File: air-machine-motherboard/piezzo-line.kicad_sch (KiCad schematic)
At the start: 8 parts, among them J3 OUT, Q1 BU407

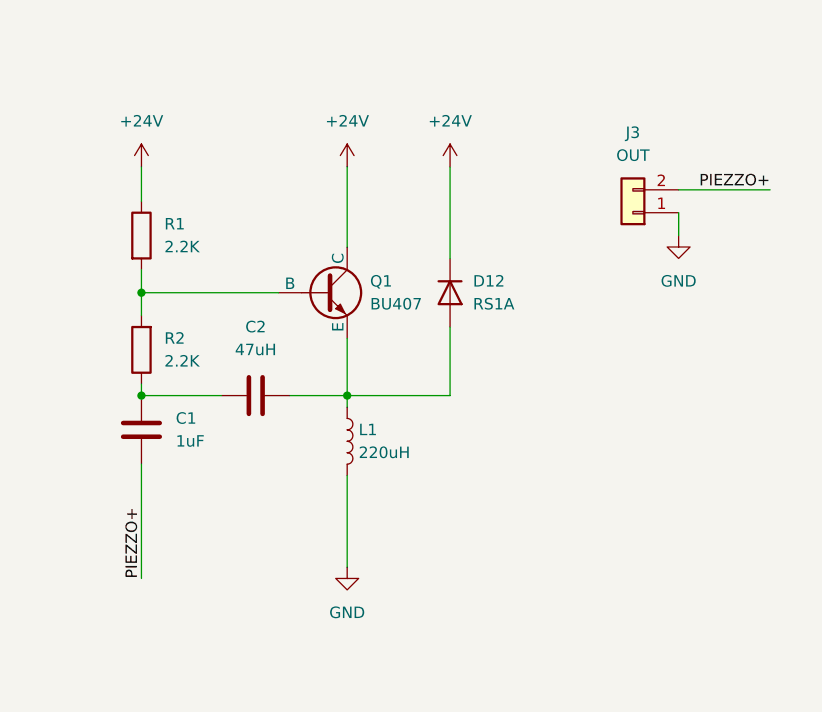
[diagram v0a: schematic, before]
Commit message: wireles air machine motherboard
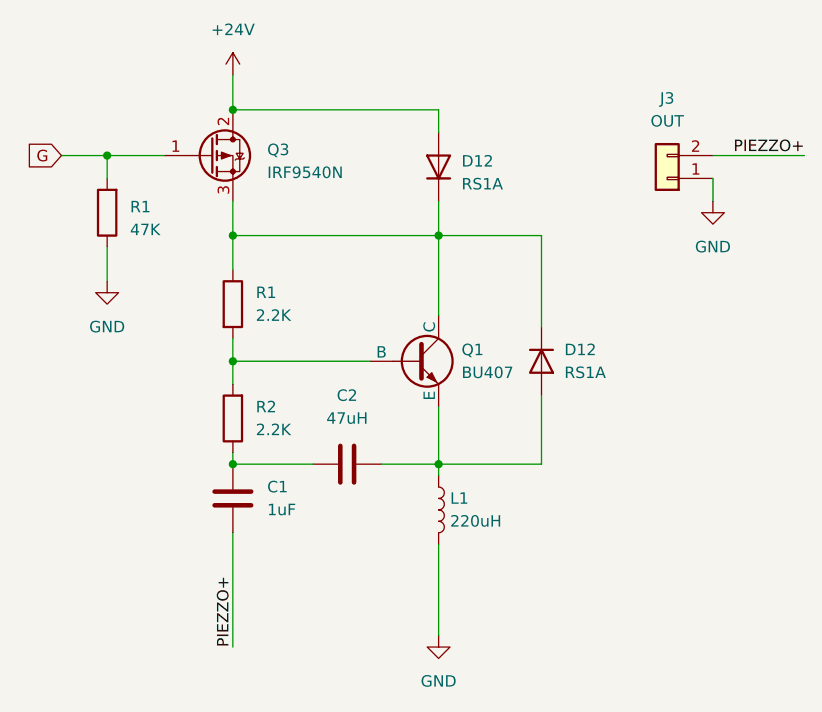
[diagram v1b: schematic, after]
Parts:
- added D12: RS1A, Diode_SMD:D_MELF, symbol Device:D
- added Q3: IRF9540N, Package_TO_SOT_THT:TO-220-3_Vertical, symbol Transistor_FET:IRF9540N
- added R1: 47K, Resistor_SMD:R_0603_1608Metric, symbol Device:R
- R1, R2: footprint Resistor_THT:R_Radial_Power_L11.0mm_W7.0mm_P5.00mm -> Resistor_SMD:R_0603_1608Metric
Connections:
- net +24V: now also D12.2 (A), Q3.2 (D); no longer D12.1 (K), Q1.1 (C), R1.1
- net GND: now also R1.1
- new net: D12.1 (K), D12.1 (K), Q1.1 (C), Q3.3 (S), R1.1
- new net G: Q3.1 (G), R1.2
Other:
- moved on the sheet: C1, C2, D12, J3, L1, Q1, R1, R2
